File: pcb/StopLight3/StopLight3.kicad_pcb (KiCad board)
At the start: 2 copper layers, 111 x 131.4 mm, 59 parts, among them J1 1935336, J2 1935336, J3 Remote Header, Q1 BT136-600, Q2 BT136-600, Q3 BT136-600, T1 FS20-600, U1 L7805, U10 MOC3021M, U2 ULN2803A, U20 MOC3021M, U30 MOC3021M

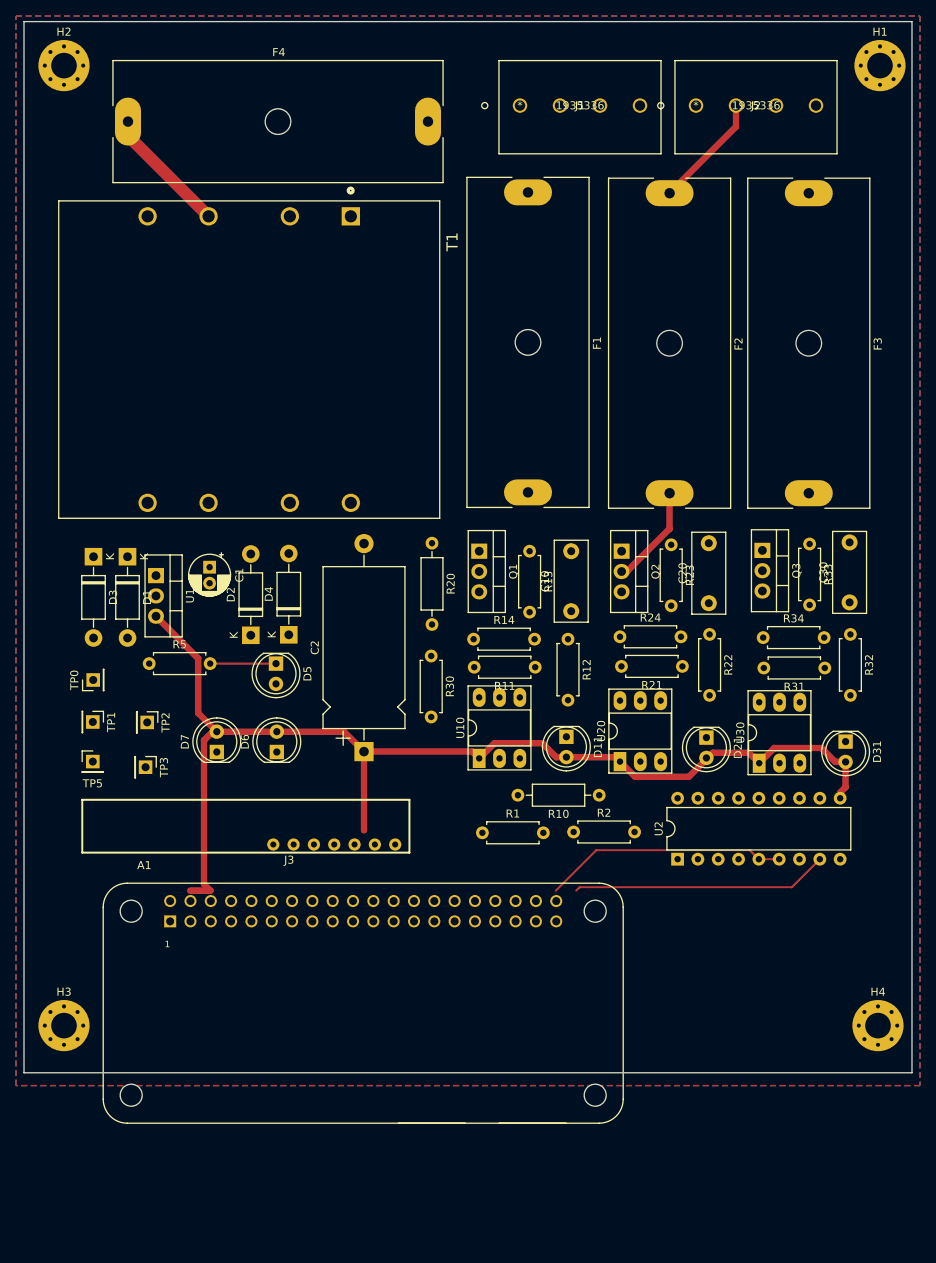
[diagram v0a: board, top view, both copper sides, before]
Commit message: PC Board design is getting close
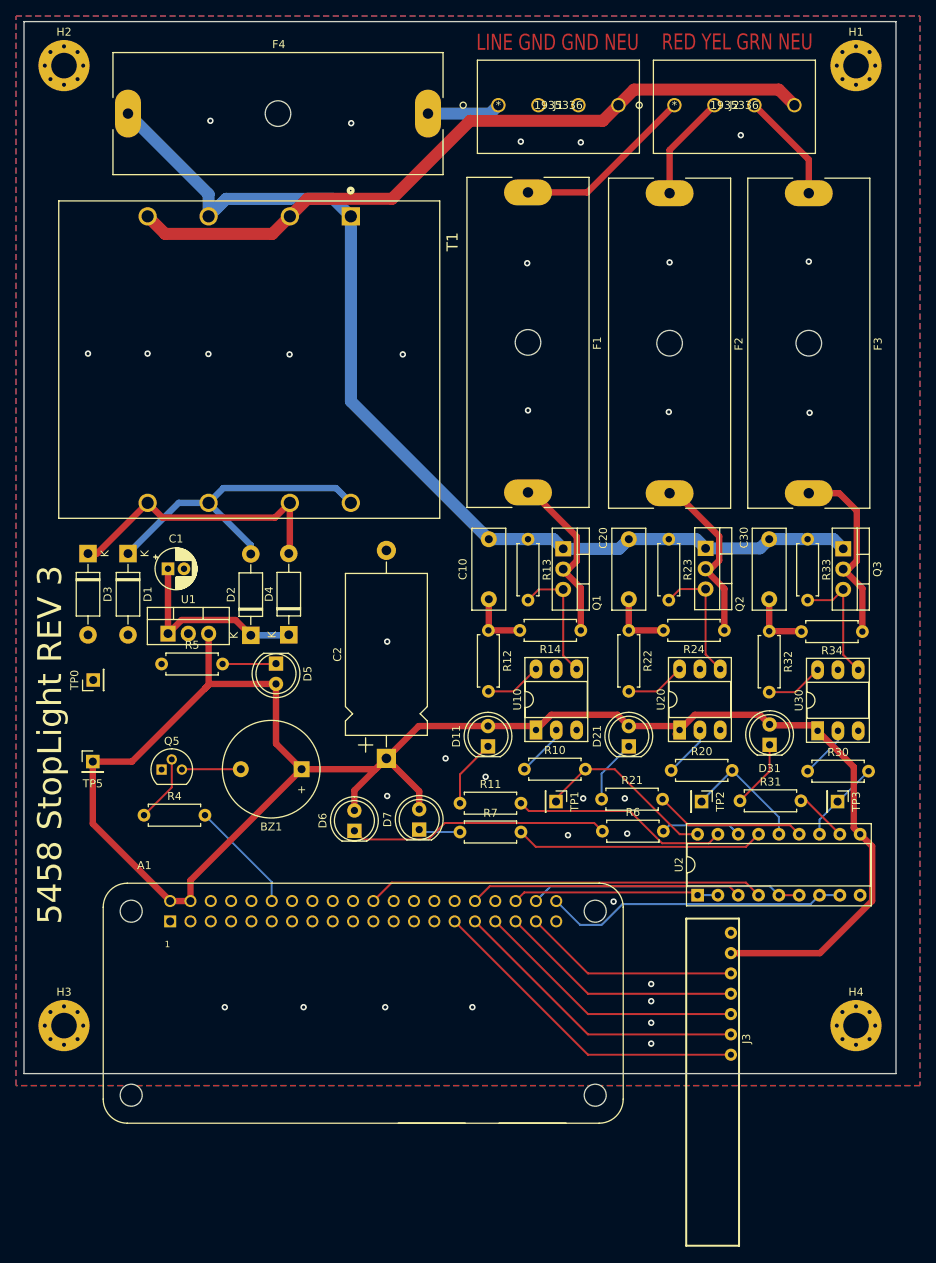
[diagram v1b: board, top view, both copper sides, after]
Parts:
- added BZ1: Buzzer, Buzzer_Beeper:Buzzer_12x9.5RM7.6, F.Cu at (59.7, 113.0)
- added Q5: 2N3904, Package_TO_SOT_THT:TO-92, F.Cu at (42.2, 113.0)
- added R4: 10R3, Resistor_THT:R_Axial_DIN0207_L6.3mm_D2.5mm_P7.62mm_Horizontal, F.Cu at (40.0, 118.7)
- R10, R20: footprint Resistor_THT:R_Axial_DIN0207_L6.3mm_D2.5mm_P10.16mm_Horizontal -> Resistor_THT:R_Axial_DIN0207_L6.3mm_D2.5mm_P7.62mm_Horizontal
- R7: renamed from R2; value 220 -> 220R
- U2: footprint Package_DIP:DIP-18_W7.62mm -> Package_DIP:DIP-18_W7.62mm_Socket
- moved TP3 86.6 mm to (126.7, 117.0)
- moved TP2 70.0 mm to (109.7, 117.0)
- moved TP1 58.7 mm to (91.5, 117.0)
- moved R30 49.2 mm to (123.0, 113.2), turned to 0 degrees
- moved R20 41.2 mm to (105.9, 113.1), turned to 0 degrees
- moved J3 40.8 mm to (109.3, 133.4), turned to 0 degrees
- moved D7 27.1 mm to (74.4, 120.5)
- moved R31 19.7 mm to (114.5, 116.9), turned to 0 degrees
- moved R21 19.4 mm to (97.2, 116.7), turned to 0 degrees
- moved R11 19.4 mm to (79.5, 117.2), turned to 0 degrees
- moved R6 15.0 mm to (97.3, 120.7)
- moved R7 14.2 mm to (79.5, 120.8)
- moved D6 13.8 mm to (66.3, 120.7)
- moved R14 13.4 mm to (94.6, 95.6), turned to 180 degrees
- moved R24 13.1 mm to (112.5, 95.6), turned to 180 degrees
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- renumbered R1 to R6
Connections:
- net Net-(A1-Pad38) renamed /YEL
- net Net-(A1-Pad40) renamed /GRN
- A1 pad 12: Net-(A1-Pad12) -> BZZ
- A1 pad 22: Net-(A1-Pad22) -> /IND2
- A1 pad 32: Net-(A1-Pad32) -> /IND1
- A1 pad 36: Net-(A1-Pad36) -> /RED
- U2 pad 1: Net-(A1-Pad12) -> /RED
- U2 pad 2: Net-(A1-Pad32) -> /RED
- U2 pad 3: Net-(A1-Pad36) -> /IND1
- U2 pad 4: Net-(A1-Pad36) -> /IND2
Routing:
- net LINE: track 16.0 -> 130.9 mm
- net NEUT: track 0.00 -> 90.0 mm
- net VCC: track 141.8 -> 223.9 mm
- net /IND2: track 0.00 -> 49.8 mm
- net /VT: track 0.00 -> 41.4 mm
- net Net-(D1-Pad1): track 0.00 -> 40.6 mm
- net /D3: track 0.00 -> 37.8 mm
- net Net-(D3-Pad1): track 0.00 -> 35.8 mm
- net /D2: track 0.00 -> 34.3 mm
- net /IND1: track 0.00 -> 34.1 mm
- net Net-(D6-Pad1): track 0.00 -> 32.7 mm
- net Net-(R7-Pad2): track 0.00 -> 31.1 mm
- net /D1: track 0.00 -> 30.7 mm
- net Net-(R11-Pad2): track 0.00 -> 27.2 mm
- net /D0: track 0.00 -> 27.1 mm
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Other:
- board size 111 x 131.4 mm -> 109 x 131.5 mm
- rule pad_to_mask_clearance: 0.05 -> 0.0508
- board text added: "5458 StopLight REV 3"
- board text added: "LINE GND GND NEU"
- board text added: "RED YEL GRN NEU"
